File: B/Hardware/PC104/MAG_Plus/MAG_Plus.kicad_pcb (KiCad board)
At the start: 2 copper layers, 96 x 89.9 mm, 106 parts, among them J1 RPi_GPIO, J2 U.FL-R-SMT(01), J3 U.FL-R-SMT(01), J4 U.FL-R-SMT(01), J5 U.FL-R-SMT(01), J6 Conn_01x12_Male, J7 Conn_01x04_Male, J8 Conn_01x04_Male, J9 Conn_01x06_Male, SW1 SW_Push, U1 Payload, U10 QPQ1906SR, U11 ISO7341C, U12 PIC16F1847-I_SO, U13 LP38693MP-3.3, U14 LP38693MP-3.3, U15 LP38693MP-5.0, U16 LP38693MP-3.3, U2 ISO1540, U3 ISO7341C, U4 AD8302, U5 AD8302, U6 AD7904BRUZ-REEL7, U7 QPQ1906SR, U8 QPQ1906SR, U9 QPQ1906SR

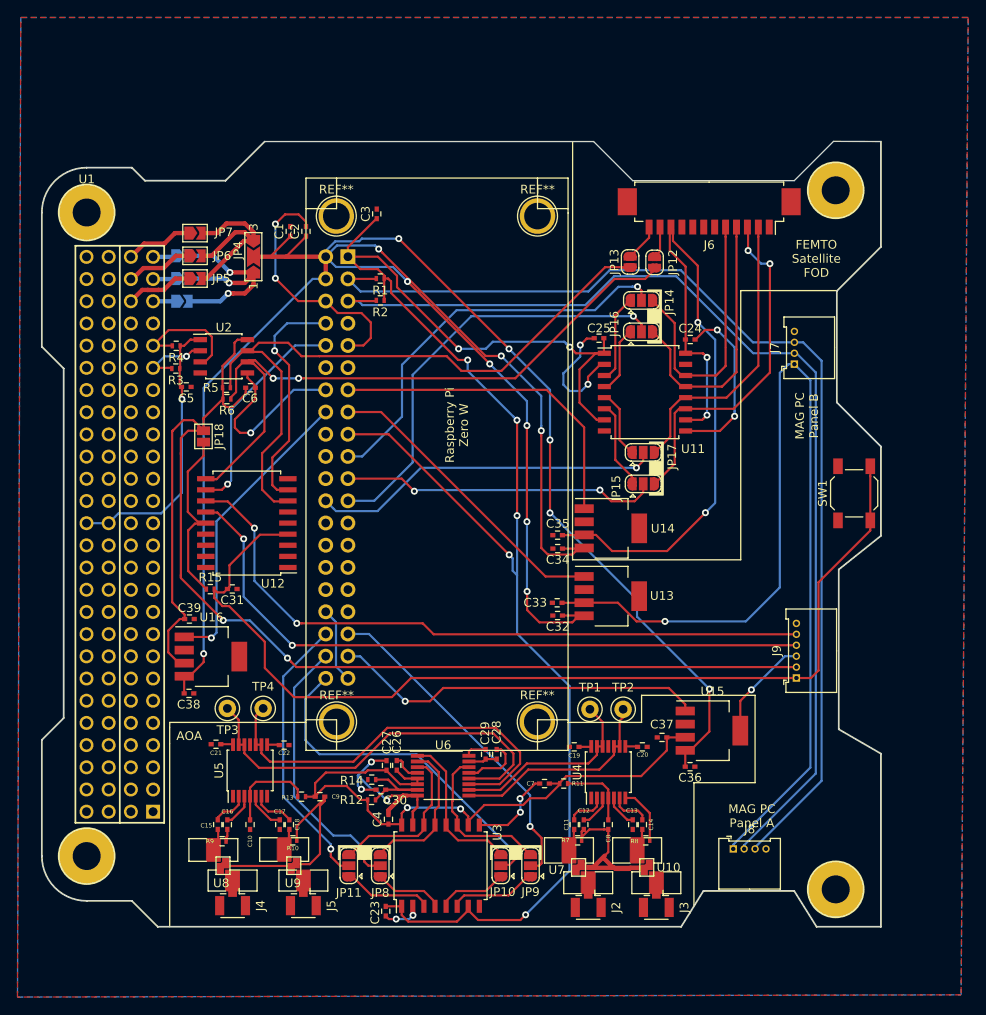
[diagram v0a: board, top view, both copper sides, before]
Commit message: PCB update
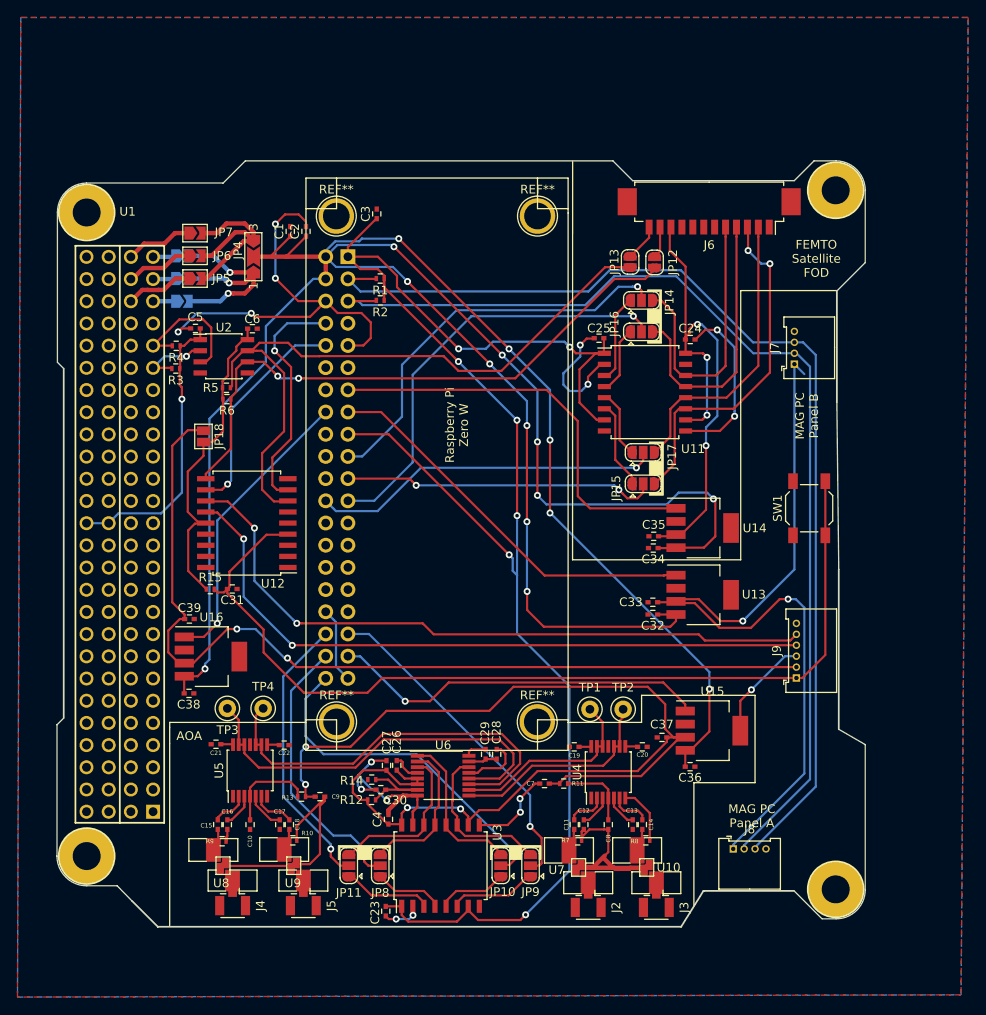
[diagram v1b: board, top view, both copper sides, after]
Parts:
- added G***: LOGO, L86:SPEL_logo, B.Cu at (178.9, 95.8)
- moved C35 11.0 mm to (175.4, 97.8)
- moved C33 11.0 mm to (175.3, 105.3)
- moved C34 10.9 mm to (175.3, 99.2)
- moved C32 10.9 mm to (175.3, 106.8)
- moved U13 10.5 mm to (181.0, 104.5)
- moved U14 10.5 mm to (181.0, 96.8)
- moved C5 6.77 mm to (123.0, 74.0), turned to 180 degrees
- moved C6 6.76 mm to (129.5, 74.0)
- moved SW1 5.43 mm to (193.2, 94.6)
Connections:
- C6 pad 1: PIC_3V3 -> PIC_3V3J
- R5 pad 1: PIC_3V3 -> PIC_3V3J
- R6 pad 1: PIC_3V3 -> PIC_3V3J
- U2 pad 8: PIC_3V3 -> PIC_3V3J
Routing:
- net AOA_5V: track 73.8 -> 136.0 mm, vias 2 -> 4
- net PIC_3V3: track 146.0 -> 105.5 mm
- net VIN: track 283.2 -> 313.6 mm, vias 14 -> 16
- net FOD_3V3: track 81.4 -> 59.4 mm
- net MAG_3V3: track 113.9 -> 93.0 mm, vias 1 -> 2
- net PIC_3V3J: track 19.8 -> 35.8 mm
- net MAG_EN: track 34.8 -> 45.3 mm
- net FOD_EN: track 38.1 -> 48.2 mm
- net PIC_SCL: track 76.1 -> 68.3 mm
- net MCLR: track 116.4 -> 109.1 mm
- net CSP_SCL: track 13.7 -> 15.3 mm
- net SAT_3V3: track 31.9 -> 33.2 mm
- net RPI_3V3: track 192.0 -> 191.1 mm
- net PIC_EN: track 34.4 -> 33.8 mm
- net FOD_SCK: track 31.2 -> 31.8 mm
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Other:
- board size 96 x 89.9 mm -> 92.5 x 86.8 mm
- board text added: "SPEL - University of Chile - 2021"
- board text added: "Sensor Board PC104 V1 Serial"
